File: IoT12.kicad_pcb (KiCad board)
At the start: 2 copper layers, 99.1 x 68.6 mm, 100 parts, among them J1 Conn_01x04_Male, Q1 2N7002, Q2 2N7002, Q3 AOD403, SW1 Rotary encoder EC11 Plum 15mm, U1 MAX809S, U2 AT24C32, U3 INA826AID, U4 INA826AID, U5 ADS1115IDGS, U6 LM393, U7 74HC125, U8 LM2596S-ADJ

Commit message: Schematic split into multiple sheets.
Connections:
- net /ESD renamed /Output/ESD
- net /IRON_- renamed /Output/IRON_-

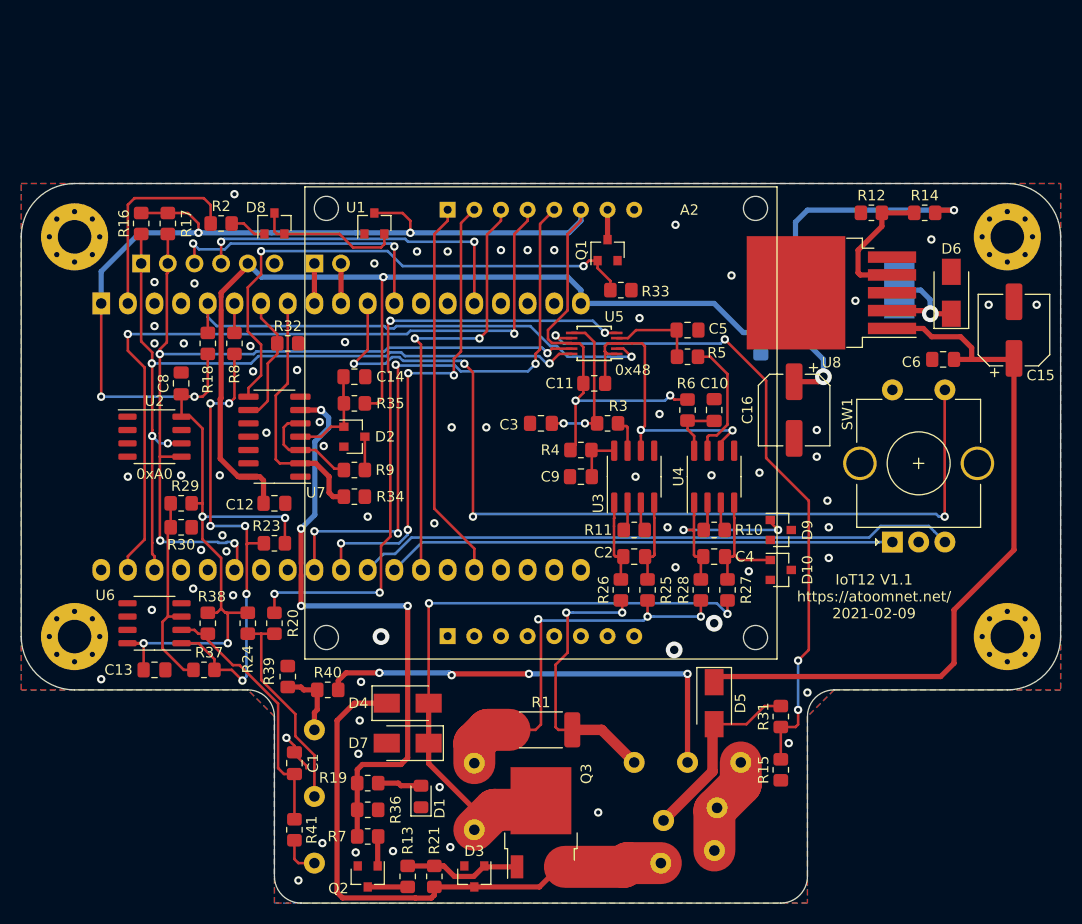
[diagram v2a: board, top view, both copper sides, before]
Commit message: V2.0 pcb.
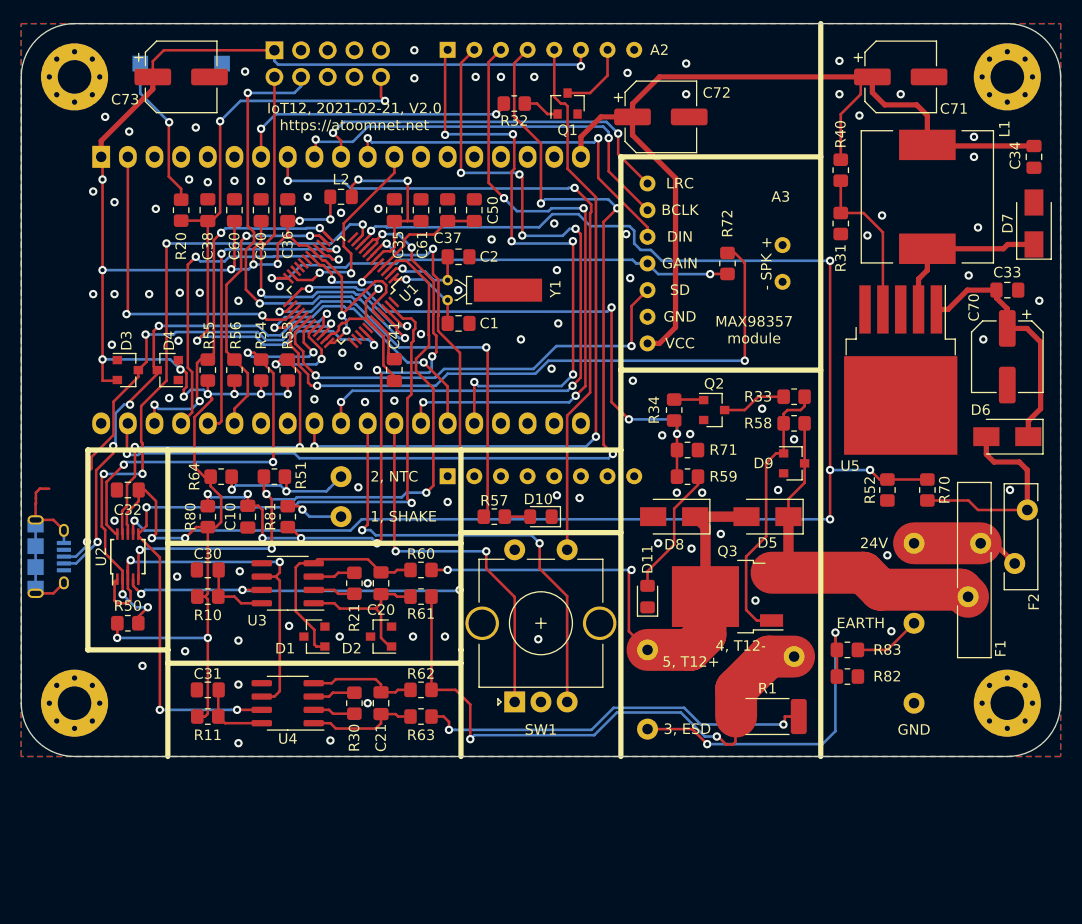
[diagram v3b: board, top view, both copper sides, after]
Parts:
- removed C11, C12, C13, C6, C7, C8, C9: 100nF, Capacitor_SMD:C_0805_2012Metric_Pad1.18x1.45mm_HandSolder
- removed C14: 10uF, Capacitor_SMD:C_0805_2012Metric_Pad1.18x1.45mm_HandSolder
- removed C15, C16: 100uF/35V, Capacitor_SMD:CP_Elec_6.3x7.7
- removed C3, C4, C5: 1nF, Capacitor_SMD:C_0805_2012Metric_Pad1.18x1.45mm_HandSolder
- removed J101, J102, J103, J105, J106, J107, J108, J109: ~, TestPoint:TestPoint_THTPad_D2.0mm_Drill1.0mm
- removed LS1: Conn_01x02_Male, Connector_PinHeader_2.54mm:PinHeader_1x02_P2.54mm_Vertical
- removed NT3: ~, NetTie-extra:NetTie-2_SMD_Pad0.25mm
- removed R12, R13: 1k, Resistor_SMD:R_0805_2012Metric_Pad1.20x1.40mm_HandSolder
- removed R14: 3k3, Resistor_SMD:R_0805_2012Metric_Pad1.20x1.40mm_HandSolder
- removed R15, R16, R17, R18, R19: 4k7, Resistor_SMD:R_0805_2012Metric_Pad1.20x1.40mm_HandSolder
- removed R2, R3, R4, R5, R6, R7, R8, R9: 100R, Resistor_SMD:R_0805_2012Metric_Pad1.20x1.40mm_HandSolder
- removed R23, R29: 10k, Resistor_SMD:R_0805_2012Metric_Pad1.20x1.40mm_HandSolder
- removed R24, R25, R26, R27, R28: 10k 0.1%, Resistor_SMD:R_0805_2012Metric_Pad1.20x1.40mm_HandSolder
- removed R35, R36, R37: 100k, Resistor_SMD:R_0805_2012Metric_Pad1.20x1.40mm_HandSolder
- removed R38, R39, R41: 1M, Resistor_SMD:R_0805_2012Metric_Pad1.20x1.40mm_HandSolder
- removed U6: LM393, Package_SO:SO-8_3.9x4.9mm_P1.27mm
- removed U7: 74HC125, Package_SO:SOIC-14_3.9x8.7mm_P1.27mm
- removed U8: LM2596S-ADJ, Package_TO_SOT_SMD:TO-263-5_TabPin3
- added A3: max98357, Module-extra:max98357, F.Cu at (17.1, -19.1)
- added C20: 1nF, Capacitor_SMD:C_0805_2012Metric_Pad1.18x1.45mm_HandSolder, F.Cu at (-15.2, 11.4)
- added C21: 1nF, Capacitor_SMD:C_0805_2012Metric_Pad1.18x1.45mm_HandSolder, F.Cu at (-15.2, 22.9)
- added C30: 100nF, Capacitor_SMD:C_0805_2012Metric_Pad1.18x1.45mm_HandSolder, F.Cu at (-31.8, 10.2)
- added C31: 100nF, Capacitor_SMD:C_0805_2012Metric_Pad1.18x1.45mm_HandSolder, F.Cu at (-31.8, 21.6)
- added C32: 100nF, Capacitor_SMD:C_0805_2012Metric_Pad1.18x1.45mm_HandSolder, F.Cu at (-39.4, 2.54)
- added C33: 100nF, Capacitor_SMD:C_0805_2012Metric_Pad1.18x1.45mm_HandSolder, F.Cu at (44.5, -16.5)
- added C34: 100nF, Capacitor_SMD:C_0805_2012Metric_Pad1.18x1.45mm_HandSolder, F.Cu at (47.0, -29.2)
- added C35: 100nF, Capacitor_SMD:C_0805_2012Metric_Pad1.18x1.45mm_HandSolder, F.Cu at (-14.0, -24.1)
- added C36: 100nF, Capacitor_SMD:C_0805_2012Metric_Pad1.18x1.45mm_HandSolder, F.Cu at (-24.1, -24.1)
- added C37: 100nF, Capacitor_SMD:C_0805_2012Metric_Pad1.18x1.45mm_HandSolder, F.Cu at (-8.89, -24.1)
- added C38: 100nF, Capacitor_SMD:C_0805_2012Metric_Pad1.18x1.45mm_HandSolder, F.Cu at (-31.8, -24.1)
- added C40: 1uF, Capacitor_SMD:C_0805_2012Metric_Pad1.18x1.45mm_HandSolder, F.Cu at (-26.7, -24.1)
- added C41: 1uF, Capacitor_SMD:C_0805_2012Metric_Pad1.18x1.45mm_HandSolder, F.Cu at (-14.0, -8.89)
- added C50: 4.7uF, Capacitor_SMD:C_0805_2012Metric_Pad1.18x1.45mm_HandSolder, F.Cu at (-6.35, -24.1)
- added C60: 10uF, Capacitor_SMD:C_0805_2012Metric_Pad1.18x1.45mm_HandSolder, F.Cu at (-29.2, -24.1)
- added C61: 10uF, Capacitor_SMD:C_0805_2012Metric_Pad1.18x1.45mm_HandSolder, F.Cu at (-11.4, -24.1)
- added C70: 100uF/35V, Capacitor_SMD:CP_Elec_6.3x7.7, F.Cu at (44.5, -10.2)
- added C71: 100uF/35V, Capacitor_SMD:CP_Elec_6.3x7.7, F.Cu at (34.3, -36.8)
- added C72: 100uF/35V, Capacitor_SMD:CP_Elec_6.3x7.7, F.Cu at (11.4, -33.0)
- added C73: 100uF/35V, Capacitor_SMD:CP_Elec_6.3x7.7, F.Cu at (-34.3, -36.8)
- added D11: Red, LED_SMD:LED_0805_2012Metric_Pad1.15x1.40mm_HandSolder, F.Cu at (10.2, 12.7)
- added J10: USB_B_Micro, Connector_USB:USB_Micro-B_Amphenol_10118194_Horizontal, B.Cu at (-46.9, 8.89)
- added J11: Conn_ARM_JTAG_SWD_10, Connector_PinHeader_2.54mm:PinHeader_2x05_P2.54mm_Vertical, B.Cu at (-25.4, -39.4)
- added J2: ~, TestPoint:TestPoint_THTPad_D2.0mm_Drill1.0mm, B.Cu at (-19.1, 1.27)
- added J3: ~, TestPoint:TestPoint_THTPad_D2.0mm_Drill1.0mm, B.Cu at (10.2, 25.3)
- added J4: ~, TestPoint:TestPoint_THTPad_D2.0mm_Drill1.0mm, B.Cu at (24.1, 18.4)
- added J5: ~, TestPoint:TestPoint_THTPad_D2.0mm_Drill1.0mm, B.Cu at (10.2, 17.8)
- added J6: ~, TestPoint:TestPoint_THTPad_D2.0mm_Drill1.0mm, B.Cu at (35.6, 7.62)
- added J7: ~, TestPoint:TestPoint_THTPad_D2.0mm_Drill1.0mm, B.Cu at (35.6, 15.2)
- added J8: ~, TestPoint:TestPoint_THTPad_D2.0mm_Drill1.0mm, B.Cu at (35.6, 22.9)
- added L2: 10uH, Inductor_SMD:L_0805_2012Metric_Pad1.15x1.40mm_HandSolder, F.Cu at (-19.1, -25.4)
- added NT4: ~, NetTie-extra:NetTie-2_SMD_Pad0.25mm, F.Cu at (18.5, 26.3)
- added NT5: ~, NetTie-extra:NetTie-2_SMD_Pad0.25mm, F.Cu at (23.5, 24.1)
- added R50: 4k7, Resistor_SMD:R_0805_2012Metric_Pad1.20x1.40mm_HandSolder, F.Cu at (-39.4, 15.2)
- added R51: 4k7, Resistor_SMD:R_0805_2012Metric_Pad1.20x1.40mm_HandSolder, F.Cu at (-25.4, 1.27)
- added R52: 4k7 1%, Resistor_SMD:R_0805_2012Metric_Pad1.20x1.40mm_HandSolder, F.Cu at (33.0, 2.54)
- added R53: 4k7, Resistor_SMD:R_0805_2012Metric_Pad1.20x1.40mm_HandSolder, F.Cu at (-24.1, -8.89)
- added R54: 4k7, Resistor_SMD:R_0805_2012Metric_Pad1.20x1.40mm_HandSolder, F.Cu at (-26.7, -8.89)
- added R55: 4k7, Resistor_SMD:R_0805_2012Metric_Pad1.20x1.40mm_HandSolder, F.Cu at (-31.8, -8.89)
- added R56: 4k7, Resistor_SMD:R_0805_2012Metric_Pad1.20x1.40mm_HandSolder, F.Cu at (-29.2, -8.89)
- added R57: 4k7, Resistor_SMD:R_0805_2012Metric_Pad1.20x1.40mm_HandSolder, F.Cu at (-4.45, 5.08)
- added R58: 4k7, Resistor_SMD:R_0805_2012Metric_Pad1.20x1.40mm_HandSolder, F.Cu at (24.1, -3.81)
- added R59: 4k7, Resistor_SMD:R_0805_2012Metric_Pad1.20x1.40mm_HandSolder, F.Cu at (14.0, 1.27)
- added R60: 10k 0.1%, Resistor_SMD:R_0805_2012Metric_Pad1.20x1.40mm_HandSolder, F.Cu at (-11.4, 10.2)
- added R61: 10k 0.1%, Resistor_SMD:R_0805_2012Metric_Pad1.20x1.40mm_HandSolder, F.Cu at (-11.4, 12.7)
- added R62: 10k 0.1%, Resistor_SMD:R_0805_2012Metric_Pad1.20x1.40mm_HandSolder, F.Cu at (-11.4, 21.6)
- added R63: 10k 0.1%, Resistor_SMD:R_0805_2012Metric_Pad1.20x1.40mm_HandSolder, F.Cu at (-11.4, 24.1)
- added R64: 10k 0.1%, Resistor_SMD:R_0805_2012Metric_Pad1.20x1.40mm_HandSolder, F.Cu at (-30.5, 1.27)
- added R70: 100k 1%, Resistor_SMD:R_0805_2012Metric_Pad1.20x1.40mm_HandSolder, F.Cu at (36.8, 2.54)
- added R71: 100k, Resistor_SMD:R_0805_2012Metric_Pad1.20x1.40mm_HandSolder, F.Cu at (14.0, -1.27)
- added R72: 100k, Resistor_SMD:R_0805_2012Metric_Pad1.20x1.40mm_HandSolder, F.Cu at (17.8, -19.1)
- added R80: 1M, Resistor_SMD:R_0805_2012Metric_Pad1.20x1.40mm_HandSolder, F.Cu at (-31.8, 5.08)
- added R81: 1M, Resistor_SMD:R_0805_2012Metric_Pad1.20x1.40mm_HandSolder, F.Cu at (-24.1, 5.08)
- added R82: 1M, Resistor_SMD:R_0805_2012Metric_Pad1.20x1.40mm_HandSolder, F.Cu at (29.2, 20.3)
- added R83: 1M, Resistor_SMD:R_0805_2012Metric_Pad1.20x1.40mm_HandSolder, F.Cu at (29.2, 17.8)
- added SW2: SW_Push, Button_Switch_SMD:SW_SPST_CK_RS282G05A3, B.Cu at (-34.3, -38.1)
- added Y1: 32768Hz, Crystal:Crystal_C26-LF_D2.1mm_L6.5mm_Horizontal_1EP_style1, F.Cu at (-8.89, -15.6)
- C1: value 100pF -> 6.7pF
- C10: value 100nF -> 100pF
- C2: value 1nF -> 6.7pF
- D1: value Red -> BAV99; footprint LED_SMD:LED_0805_2012Metric_Pad1.15x1.40mm_HandSolder -> Package_TO_SOT_SMD:SOT-23
- D10: value BAV99 -> Amber; footprint Package_TO_SOT_SMD:SOT-23 -> LED_SMD:LED_0805_2012Metric_Pad1.15x1.40mm_HandSolder
- D3: value BZX84C18 -> BAV99; footprint Diode_SMD:D_SOT-23_ANK -> Package_TO_SOT_SMD:SOT-23
- D4: value SS14 -> BAV99; footprint Diode_SMD:D_SMA -> Package_TO_SOT_SMD:SOT-23
- D5: value SS34 -> SS14
- D8: value BAV99 -> SS34; footprint Package_TO_SOT_SMD:SOT-23 -> Diode_SMD:D_SMA
- D9: value BAV99 -> BZX84C18; footprint Package_TO_SOT_SMD:SOT-23 -> Diode_SMD:D_SOT-23_ANK
- F1: value 0.5A/30V -> 2.5A/30V; footprint Fuse:Fuse_Bourns_MF-RG400 -> Fuse:Fuse_Bourns_MF-RG1000; moved to F.Cu
- F2: value 2.5A/30V -> 0.5A/30V; footprint Fuse:Fuse_Bourns_MF-RG1000 -> Fuse:Fuse_Bourns_MF-RG400; moved to F.Cu
- J1: value Conn_01x04_Male -> ~; footprint Connector_PinHeader_2.54mm:PinHeader_1x06_P2.54mm_Vertical -> TestPoint:TestPoint_THTPad_D2.0mm_Drill1.0mm
- L1: moved to F.Cu
- Q1, Q2: value 2N7002 -> MMBT2222
- R10: value 470R 1% -> 100R
- R11: value 1k 1% -> 100R
- R20: value 4k7 -> 470R
- R21: value 4k7 -> 470R 1%
- R30: value 33k -> 1k 1%
- R31, R32, R33, R34: value 100k -> 1k
- R40: value 1M -> 3k3
- U1: value MAX809S -> ATSAMD21G; footprint Package_TO_SOT_SMD:SOT-23 -> Package_QFP:TQFP-48_7x7mm_P0.5mm
- U2: value AT24C32 -> ADS1115IDGS; footprint Package_SO:SO-8_3.9x4.9mm_P1.27mm -> Package_SO:TSSOP-10_3x3mm_P0.5mm
- U5: value ADS1115IDGS -> LM2596S-ADJ; footprint Package_SO:TSSOP-10_3x3mm_P0.5mm -> Package_TO_SOT_SMD:TO-263-5_TabPin3
- moved H2 90.2 mm to (44.5, -36.8)
- moved H3 89.1 mm to (-44.5, 22.9)
- moved D7 77.6 mm to (47.0, -22.9), turned to 90 degrees
- moved R40 69.6 mm to (28.6, -27.9), turned to 270 degrees
- moved D3 58.5 mm to (-39.4, -8.89), turned to 0 degrees
- moved Q2 55.4 mm to (16.5, -5.08), turned to 0 degrees
- moved H4 53.3 mm to (-44.5, -36.8)
- moved NT1 52.9 mm to (-39.4, 9.65), turned to 270 degrees
- moved NT2 51.9 mm to (-48.1, 3.56), turned to 90 degrees
- moved R10 48.7 mm to (-31.8, 12.7)
- moved F2 48.5 mm to (46.4, 4.45), turned to 270 degrees
- moved R31 47.3 mm to (28.6, -22.9)
- moved D8 47.2 mm to (12.7, 5.08), turned to 180 degrees
- moved U4 46.0 mm to (-24.1, 22.9), turned to 180 degrees
- moved C10 45.6 mm to (-27.9, 5.08), turned to 270 degrees
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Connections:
- net Net-(F1-Pad2) renamed /Power/24V_DC
- A1 pad 10: Net-(A1-Pad10) -> I2S_WS
- A1 pad 11: ROT_SW -> I2S_DATA
- A1 pad 12: IO14 -> HEAT_INT
- A1 pad 15: IO13 -> Net-(A1-Pad15)
- A1 pad 2: ~RESET -> ESP32_EN
- A1 pad 25: Net-(A1-Pad25) -> ESP32_IO0
- A1 pad 33: SDA -> ESP32_SDA
- A1 pad 34: Net-(A1-Pad34) -> ESP32_RXD
- A1 pad 35: Net-(A1-Pad35) -> ESP32_TXD
- A1 pad 36: SCL -> ESP32_SCL
- A1 pad 5: ADC_RDY -> Net-(A1-Pad5)
- A1 pad 6: SHAKE -> Net-(A1-Pad6)
- A1 pad 8: PWM_HEAT -> ROT_SW
- A1 pad 9: Net-(A1-Pad9) -> I2S_BCK
- C1 pad 1: Net-(C1-Pad1) -> /Brain/XIN32
- C10 pad 1: Net-(C10-Pad1) -> AIN_COMP
- C2 pad 1: Net-(C2-Pad1) -> /Brain/XOUT32
- C2 pad 2: Net-(C2-Pad2) -> GND
- D1 pad 1: GND -> Net-(C20-Pad1)
- D1 pad 2: Net-(D1-Pad2) -> GND
- D10 pad 1: Net-(C4-Pad1) -> GND
- D10 pad 2: GND -> Net-(D10-Pad2)
- D2 pad 1: Net-(C14-Pad1) -> Net-(C20-Pad2)
- D2 pad 2: Net-(D2-Pad2) -> GND
- D2 pad 3: Net-(D2-Pad3) -> GND
- D3 pad 1: +24V -> GND
- D3 pad 2: Net-(D3-Pad2) -> +3V3
- D4 pad 1: +24V -> GND
- D4 pad 2: IRON_+ -> +3V3
- D5 pad 1: Net-(C15-Pad1) -> +24V
- D5 pad 2: Net-(D5-Pad2) -> IRON_+
- D6 pad 1: Net-(D6-Pad1) -> /Power/24V_DC_SW
- D6 pad 2: GND -> Net-(D6-Pad2)
- D7 pad 1: IRON_+ -> Net-(D7-Pad1)
- D8 pad 1: Net-(D8-Pad1) -> IRON_+
- D8 pad 2: Net-(D8-Pad2) -> GND
- D9 pad 1: Net-(C4-Pad2) -> +24V
- D9 pad 2: GND -> /Output/GATE
- F1 pad 1: Net-(D5-Pad2) -> +24V
- F2 pad 1: +24V -> Net-(D6-Pad2)
- J1 pad 1: SCL -> Net-(J1-Pad1)
- L1 pad 1: Net-(D6-Pad1) -> Net-(D7-Pad1)
- NT2 pad 1: /Output/IRON_- -> Net-(J10-Pad5)
- NT2 pad 2: NEAR_RSENSE_+ -> GND
- Q2 pad 1: SAFE_PWM_HEAT -> Net-(Q2-Pad1)
- Q3 pad 1: Net-(D3-Pad2) -> /Output/GATE
- R10 pad 1: Net-(R10-Pad1) -> Net-(C30-Pad1)
- R10 pad 2: Net-(R10-Pad2) -> +3V3
- R11 pad 1: Net-(R11-Pad1) -> Net-(C31-Pad1)
- R11 pad 2: Net-(R11-Pad2) -> +3V3
- R20 pad 1: NTC -> Net-(R20-Pad1)
- R20 pad 2: Net-(J105-Pad1) -> HEAT_~RESET
- R21 pad 1: +24V -> Net-(R21-Pad1)
- R21 pad 2: Net-(D3-Pad2) -> Net-(R21-Pad2)
- R30 pad 1: GND -> Net-(R30-Pad1)
- R30 pad 2: Net-(R29-Pad1) -> Net-(R30-Pad2)
- R31 pad 1: VIN -> GND
- R31 pad 2: Net-(D5-Pad2) -> Net-(R31-Pad2)
- R32 pad 1: LCD_LED -> Net-(Q1-Pad1)
- R32 pad 2: GND -> LCD_LED
- R33 pad 1: Net-(Q1-Pad1) -> /Output/GATE
- R33 pad 2: GND -> Net-(Q2-Pad3)
- R34 pad 1: PWM_HEAT -> Net-(Q2-Pad1)
- R34 pad 2: GND -> PWM_HEAT
- R40 pad 1: /Output/ESD -> +5V
- R40 pad 2: Earth -> Net-(R31-Pad2)
- U1 pad 1: GND -> /Brain/XIN32
- U1 pad 2: Net-(D8-Pad2) -> /Brain/XOUT32
- U1 pad 3: +3V3 -> NTC
- U2 pad 1: Net-(U2-Pad1) -> GND
- U2 pad 2: Net-(U2-Pad2) -> ADC_RDY
- U2 pad 3: Net-(U2-Pad3) -> GND
- U2 pad 4: GND -> TEMP
- U2 pad 5: SDA -> NTC
- U2 pad 6: SCL -> IRON_POWER
- U2 pad 7: Net-(U2-Pad7) -> VIN
- U3 pad 1: Net-(C2-Pad2) -> Net-(C20-Pad2)
- U3 pad 2: Net-(R11-Pad2) -> Net-(R21-Pad2)
- U3 pad 3: Net-(R11-Pad1) -> Net-(R21-Pad1)
- U3 pad 4: Net-(C2-Pad1) -> Net-(C20-Pad1)
- U3 pad 7: Net-(R3-Pad2) -> TEMP
- U3 pad 8: Net-(C9-Pad1) -> Net-(C30-Pad1)
- U4 pad 1: Net-(C4-Pad2) -> Net-(C21-Pad2)
- U4 pad 2: Net-(R10-Pad2) -> Net-(R30-Pad2)
- U4 pad 3: Net-(R10-Pad1) -> Net-(R30-Pad1)
- U4 pad 4: Net-(C4-Pad1) -> Net-(C21-Pad1)
- U4 pad 7: Net-(R5-Pad2) -> IRON_POWER
- U4 pad 8: Net-(C10-Pad1) -> Net-(C31-Pad1)
- U5 pad 1: GND -> /Power/24V_DC_SW
- U5 pad 2: ADC_RDY -> Net-(D7-Pad1)
- U5 pad 4: TEMP -> Net-(R31-Pad2)
- U5 pad 5: NTC -> GND
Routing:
- net VIN: track 63.5 -> 151.5 mm, vias 4 -> 6
- net SDA: track 81.5 -> 0.00 mm, vias 4 -> 0
- net SCL: track 76.9 -> 0.00 mm, vias 4 -> 0
- net Net-(C15-Pad1): track 70.2 -> 0.00 mm
- net TEMP: track 8.58 -> 74.8 mm, vias 0 -> 5
- net AIN_COMP: track 0.00 -> 65.8 mm, vias 0 -> 9
- net HEAT_~RESET: track 0.00 -> 63.6 mm, vias 0 -> 4
- net IRON_POWER: track 14.7 -> 76.5 mm, vias 2 -> 4
- net I2S_GAIN1: track 0.00 -> 61.6 mm, vias 0 -> 2
- net Net-(R19-Pad1): track 58.3 -> 0.00 mm, vias 4 -> 0
- net Net-(Q1-Pad1): track 51.6 -> 3.54 mm, vias 2 -> 0
- net +3V3: track 181.0 -> 228.5 mm, vias 10 -> 21
- net /Brain/USB-: track 0.00 -> 47.1 mm, vias 0 -> 5
- net I2S_GAIN0: track 0.00 -> 46.5 mm, vias 0 -> 2
- net SWCLK: track 0.00 -> 46.4 mm, vias 0 -> 3
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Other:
- board size 99.1 x 68.6 mm -> 99.1 x 69.8 mm
- board text added: "- SPK +"
- board text added: "1, SHAKE"
- board text added: "2, NTC"
- board text added: "3, ESD"
- board text added: "4, T12-"
- board text added: "5, T12+"
- board text added: "ESP32-DevKitC module"
- board text added: "IoT12, 2021-02-21, V2.0 https://atoomnet.net"
- board text added: "MAX98357 module"
- board text added: "RESET SAMD21"
- board text added: "SWD SAMD21"
- board text added: "USB SAMD21"
- board text removed: "0x48"
- board text removed: "0xA0"
- board text removed: "1, blue, shake."
- board text removed: "2, white, NTC."
- board text removed: "3, green, earth."
- board text removed: "4, black, ground."
- board text removed: "5, red, +."
- board text removed: "5V"
- board text removed: "IO13"
- board text removed: "IO14"
- board text removed: "IoT12 V1.1 https://atoomnet.net/ 2021-02-09"
- board text removed: "Piezo"
- board text removed: "Power supply connector"
- board text removed: "SCL"
- board text removed: "SDA"
- board text removed: "Solder iron connector"
